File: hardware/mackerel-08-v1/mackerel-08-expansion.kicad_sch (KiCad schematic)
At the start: 2 parts, among them J5 Conn_02x10_Odd_Even, J8 Conn_02x20_Odd_Even

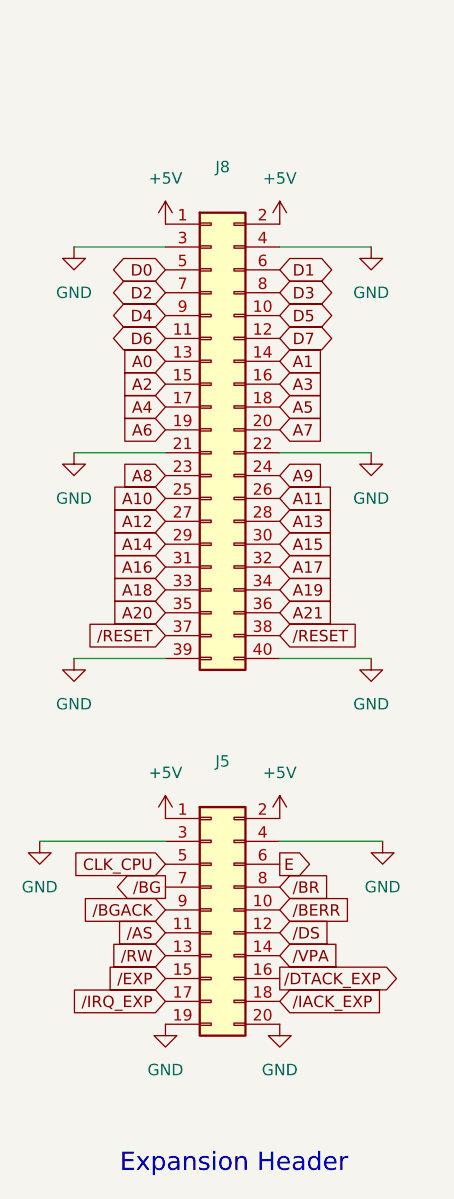
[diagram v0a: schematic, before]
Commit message: Mack-08 rev 1.1 routed
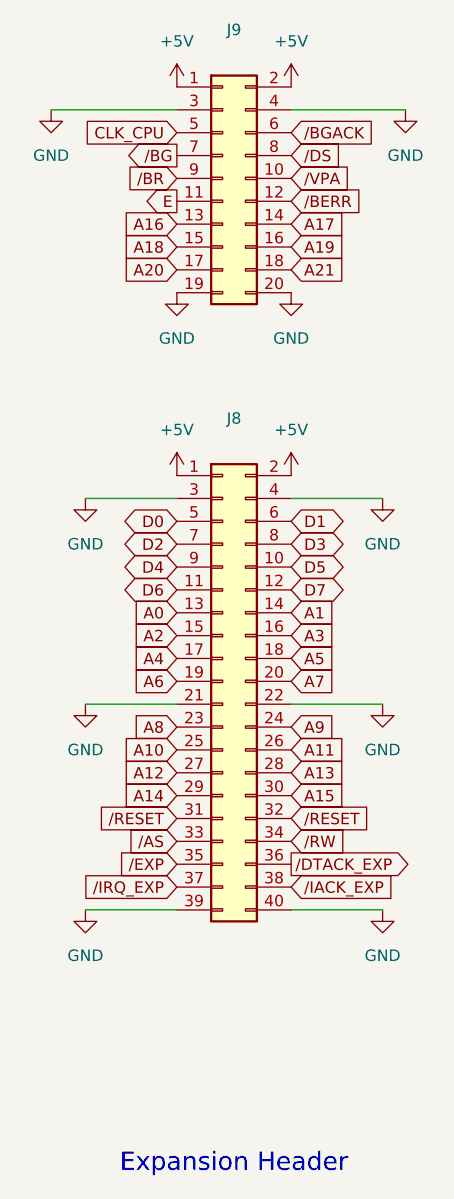
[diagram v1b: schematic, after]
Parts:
- renumbered J5 to J9
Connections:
- net A16: now also J9.13 (Pin_13); no longer J8.31 (Pin_31)
- net A17: now also J9.14 (Pin_14); no longer J8.32 (Pin_32)
- net A18: now also J9.15 (Pin_15); no longer J8.33 (Pin_33)
- net A19: now also J9.16 (Pin_16); no longer J8.34 (Pin_34)
- net A20: now also J9.17 (Pin_17); no longer J8.35 (Pin_35)
- net A21: now also J9.18 (Pin_18); no longer J8.36 (Pin_36)
- net E: now also J9.11 (Pin_11); no longer J9.6 (Pin_6)
- net /AS: now also J8.33 (Pin_33); no longer J9.11 (Pin_11)
- net /BERR: now also J9.12 (Pin_12); no longer J9.10 (Pin_10)
- net /BGACK: now also J9.6 (Pin_6); no longer J9.9 (Pin_9)
- net /BR: now also J9.9 (Pin_9); no longer J9.8 (Pin_8)
- net /DS: now also J9.8 (Pin_8); no longer J9.12 (Pin_12)
- net /DTACK_EXP: now also J8.36 (Pin_36); no longer J9.16 (Pin_16)
- net /EXP: now also J8.35 (Pin_35); no longer J9.15 (Pin_15)
- net /IACK_EXP: now also J8.38 (Pin_38); no longer J9.18 (Pin_18)
- net /IRQ_EXP: now also J8.37 (Pin_37); no longer J9.17 (Pin_17)
- net /RESET: now also J8.31 (Pin_31), J8.32 (Pin_32); no longer J8.37 (Pin_37), J8.38 (Pin_38)
- net /RW: now also J8.34 (Pin_34); no longer J9.13 (Pin_13)
- net /VPA: now also J9.10 (Pin_10); no longer J9.14 (Pin_14)
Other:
- moved on the sheet: J8, J9

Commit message: Add Mackerel-08 BOM list
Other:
- title: Mackerel-08 SBC v1 -> Mackerel-08 SBC v1.1
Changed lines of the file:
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@@
 	(paper "A")
 	(title_block
-		(title "Mackerel-08 SBC v1")
+		(title "Mackerel-08 SBC v1.1")
 		(date "2024-08-22")
 		(rev "1.1")
